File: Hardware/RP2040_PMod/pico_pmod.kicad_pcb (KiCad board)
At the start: 2 copper layers, 50 x 37 mm, 45 parts, among them J1 Conn_02x06_Odd_Even, J2 Conn_02x06_Odd_Even, J3 Conn_02x06_Odd_Even, J4 USB_C_Receptacle_USB2.0, J5 Conn_01x04, SW1 SW_Push, SW2 SW_Push, U1 RP2040, U2 W25Q128JVS, U3 NCP1117-3.3_SOT223, Y1 12MHz

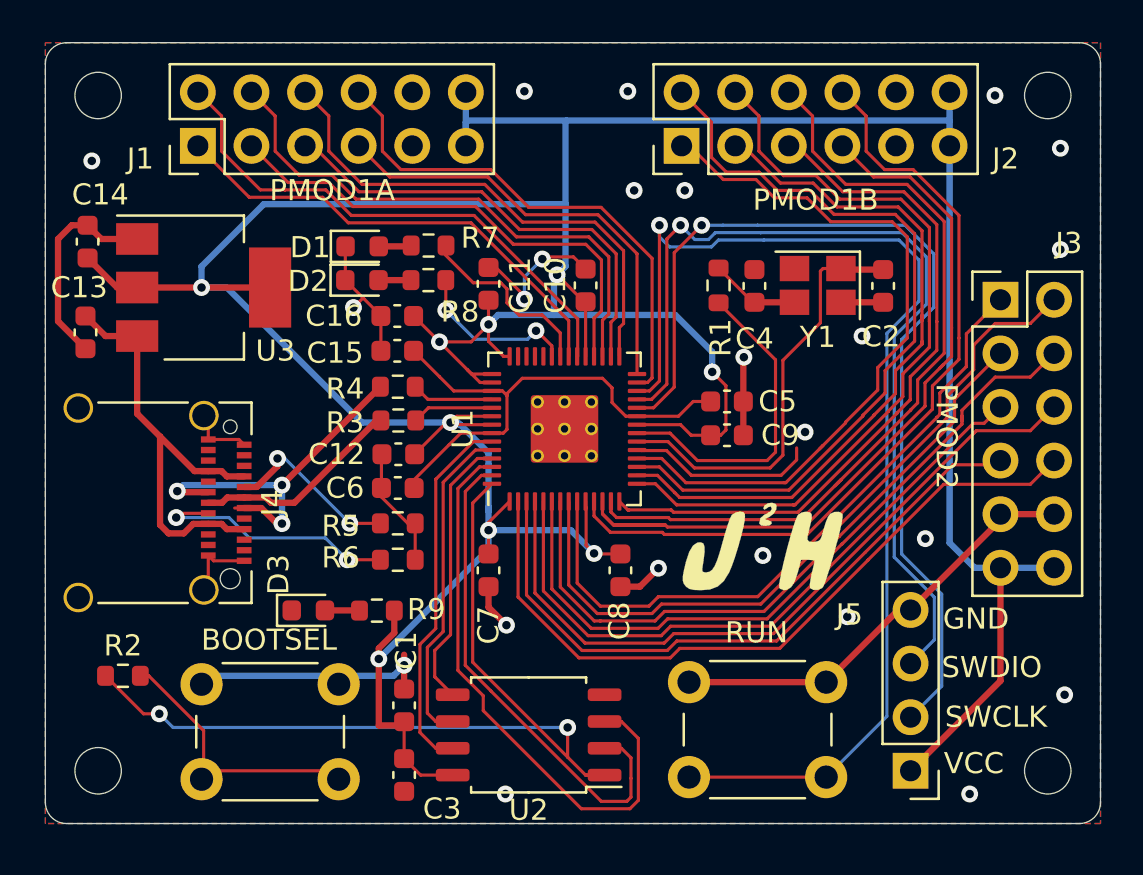
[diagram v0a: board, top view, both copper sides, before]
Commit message: update to kicad 6.0
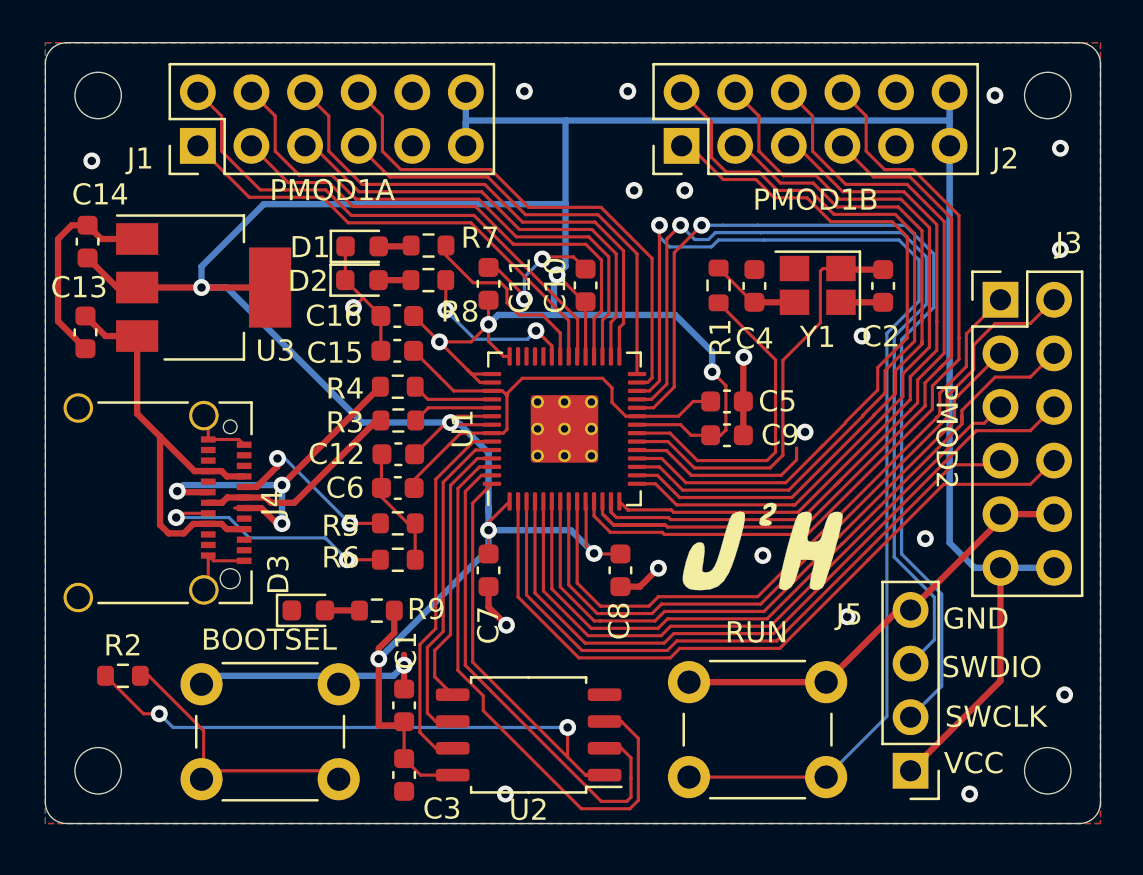
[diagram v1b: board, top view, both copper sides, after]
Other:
- net class Default removed
